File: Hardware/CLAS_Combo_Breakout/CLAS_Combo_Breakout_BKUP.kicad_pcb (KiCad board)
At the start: 4 copper layers, 60 x 60 mm, 70 parts, among them J1 USB_C_Receptacle_USB2.0, J2 USB_C_Receptacle_USB2.0, J3 Conn_SMA, U1 USBLC6-2P6, U10 NT1191GEAE3S, U2 ZED-F9P, U3 NEO-D9C-00B, U4 USBLC6-2P6, U5 LMV331, U6 AP2112K-3.3, U7 DSS20200, U8 PD0922J5050S2HF, U9 F2933NBGP

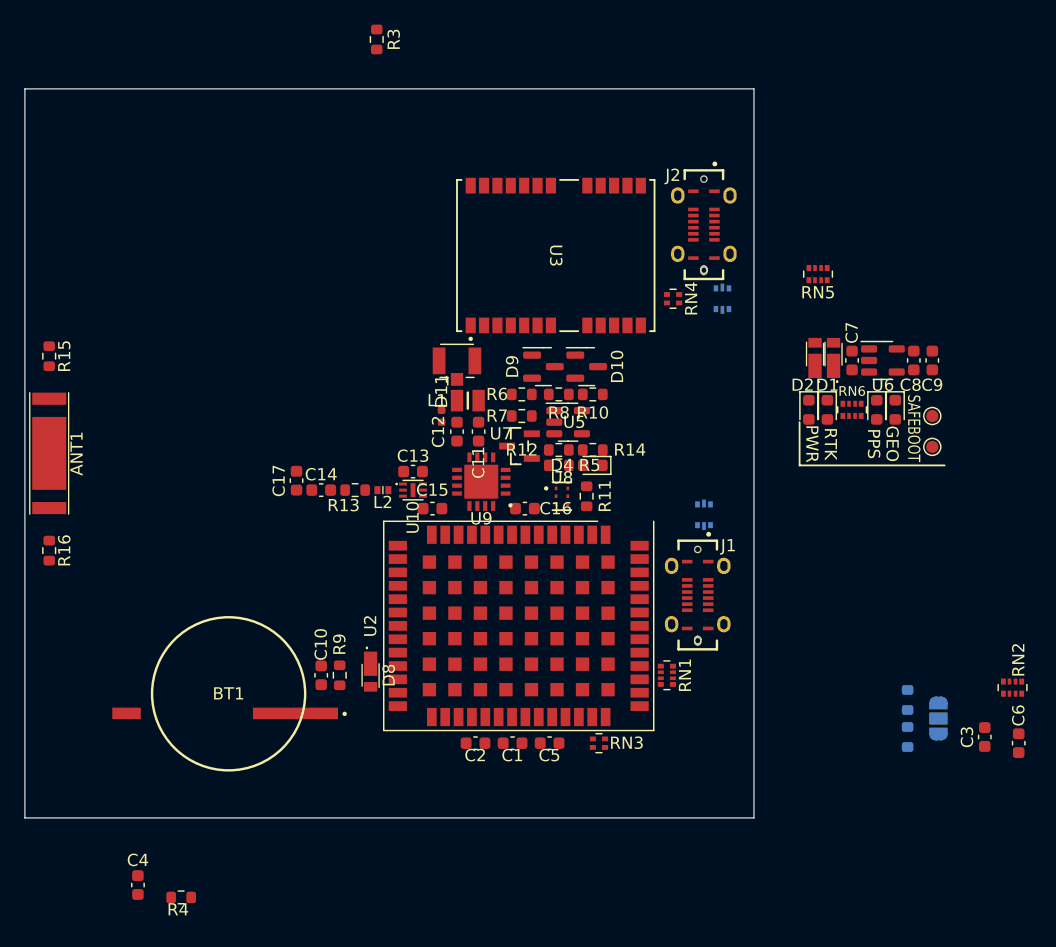
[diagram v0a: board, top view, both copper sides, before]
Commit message: 配線
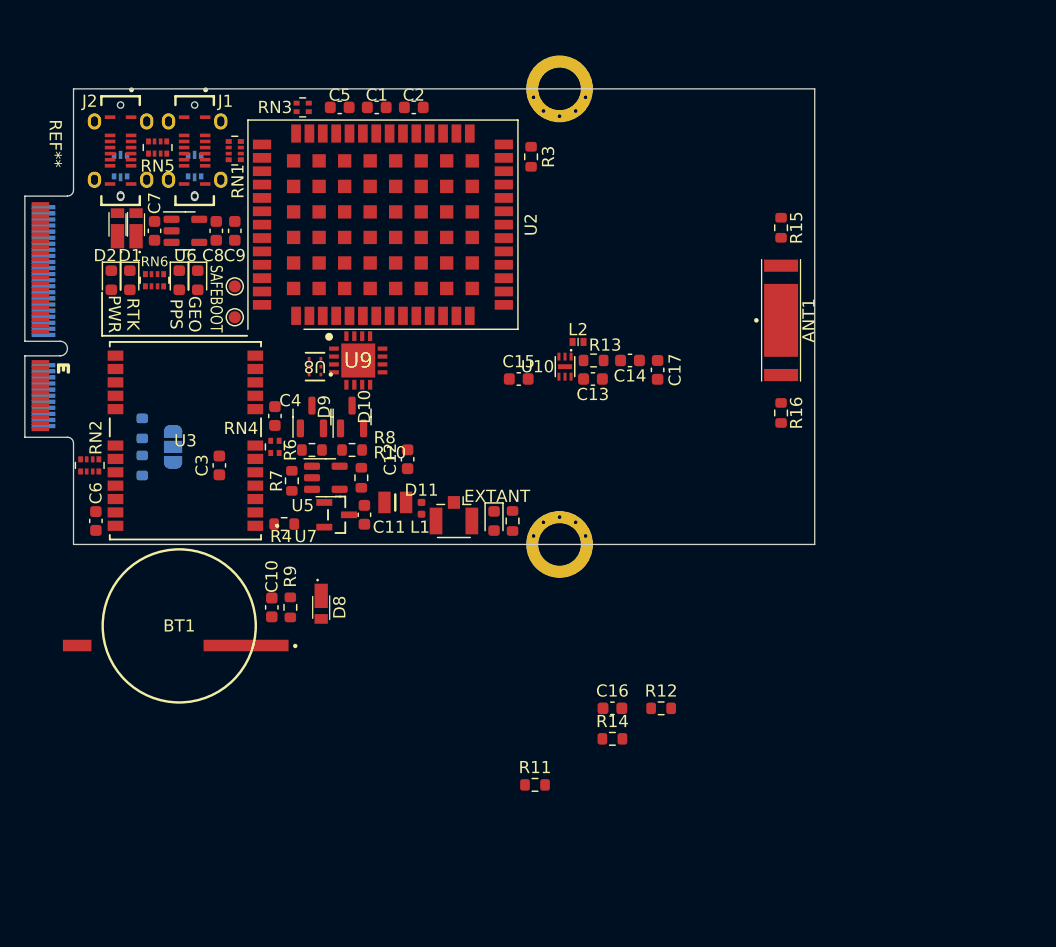
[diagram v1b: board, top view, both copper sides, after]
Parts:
- added REF**: MicroMod_FunctionCard, MicroMod_KiCad:MicroMod_FunctionCard, F.Cu at (100.0, 90.0)
- ANT1: value GGBLA125A -> GGBLA.125.A
- L2: value LQW15CNR20J00B -> LQW15AN9N5G00D
- U9: value F2933NBGP -> QFN65P400X400X100-17N-D
- moved C6 78.1 mm to (105.8, 125.6)
- moved RN2 78.1 mm to (105.3, 121.0)
- moved C3 66.8 mm to (116.0, 121.0)
- moved JP1 66.8 mm to (112.2, 119.5)
- moved R1 66.8 mm to (109.7, 121.0)
- moved R2 66.8 mm to (109.7, 117.9)
- moved R16 61.3 mm to (162.2, 116.7)
- moved ANT1 61.2 mm to (162.2, 109.0)
- moved R15 61.2 mm to (162.2, 101.4)
- moved D7 58.4 mm to (112.7, 105.7)
- moved C7 58.4 mm to (110.7, 101.7)
- moved C8 58.4 mm to (115.7, 101.7)
- moved C9 58.4 mm to (117.3, 101.7)
- moved D1 58.4 mm to (109.1, 101.2)
- moved D2 58.4 mm to (107.6, 101.2)
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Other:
- board size 60 x 60 mm -> 65 x 37.5 mm
- board text added: "0.8mm PCB"
- board text added: "Chamfered Edge"
- board text added: "EXTANT"
- board text added: "Route Out"
